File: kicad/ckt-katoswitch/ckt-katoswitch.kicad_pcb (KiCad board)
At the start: 2 copper layers, 76.2 x 63.5 mm, 50 parts, among them J1 SM04B-SRSS, J10 SM04B-SRSS, J11 Conn_AVR_TagConnect_TC2030, J2 SM04B-SRSS, J3 SM04B-SRSS, J4 SM04B-SRSS, J5 SM04B-SRSS, J6 SM04B-SRSS, J7 SM04B-SRSS, J8 SM04B-SRSS, J9 SM04B-SRSS, Q1 ZXMS6004FF, SW1 SW_DIP_x05, U1 AP7381-33Y, U2 ATtiny861A-S

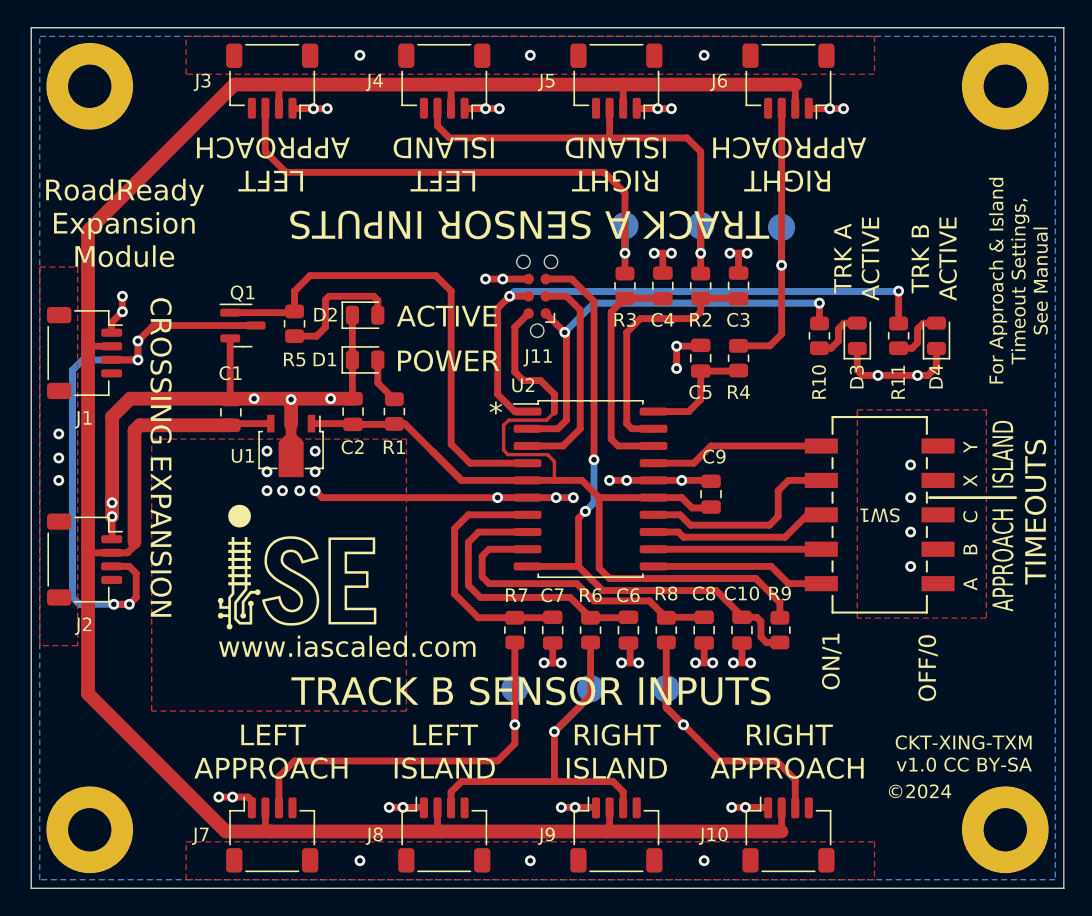
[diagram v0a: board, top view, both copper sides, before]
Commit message: Initial cut at PCB
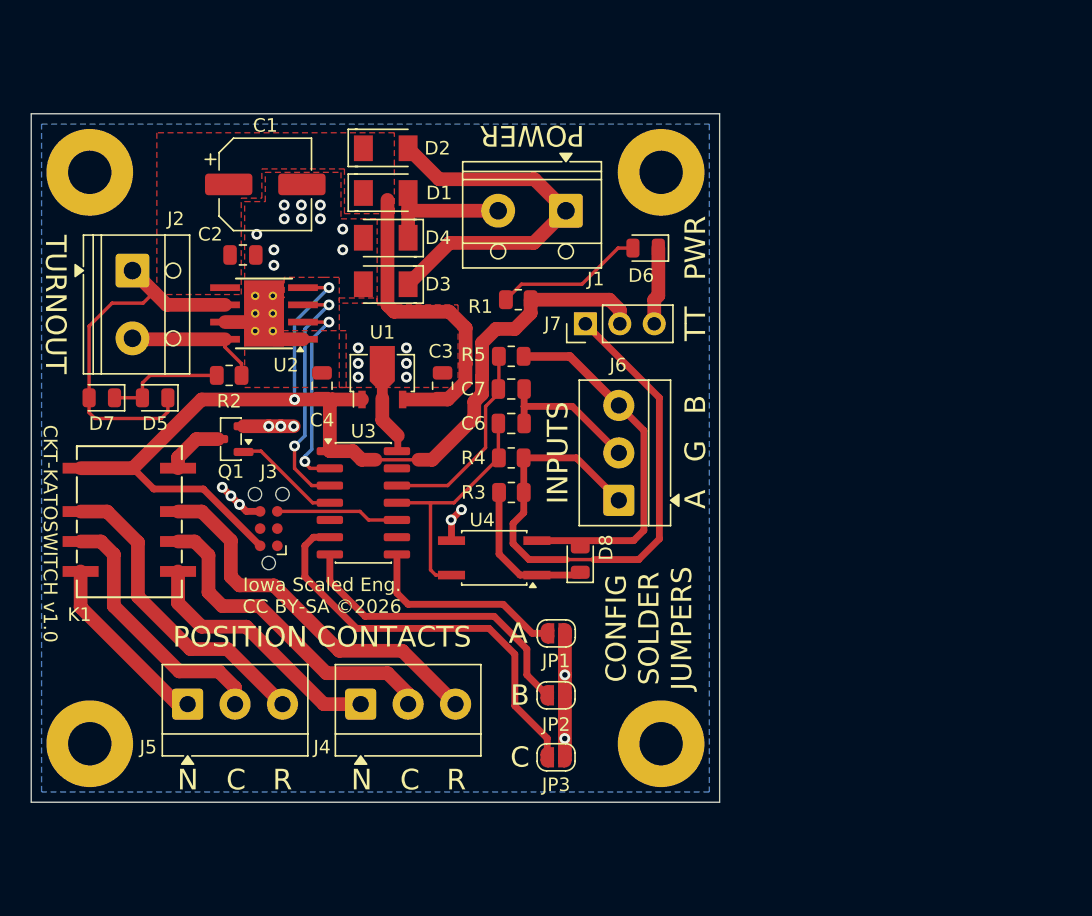
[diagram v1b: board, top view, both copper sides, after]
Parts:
- removed C10, C5, C8: 1uF, Capacitor_SMD:C_0805_2012Metric
- removed C9: 0.1uF, Capacitor_SMD:C_0805_2012Metric
- removed J10, J8, J9: SM04B-SRSS, Connector_JST:JST_SH_SM04B-SRSS-TB_1x04-1MP_P1.00mm_Horizontal
- removed J11: Conn_AVR_TagConnect_TC2030, Connector:Tag-Connect_TC2030-IDC-NL_2x03_P1.27mm_Vertical
- removed R10, R11, R6, R7, R8: 1k, Resistor_SMD:R_0805_2012Metric
- removed R9: 10k, Resistor_SMD:R_0805_2012Metric
- removed SW1: SW_DIP_x05, ISE_UltraLibrarian:CST_219SMT
- removed TP1, TP2, TP3, TP4, TP5, TP6: TestPoint, TestPoint:TestPoint_Pad_D2.0mm
- added D5: AMBER, LED_SMD:LED_0805_2012Metric, F.Cu at (34.5, 46.4)
- added D6: GREEN LED, LED_SMD:LED_0805_2012Metric, F.Cu at (70.7, 35.3)
- added D7: BLUE, LED_SMD:LED_0805_2012Metric, F.Cu at (30.6, 46.4)
- added D8: AMBER, LED_SMD:LED_0805_2012Metric, F.Cu at (65.9, 58.3)
- added JP1: SolderJumper_2_Open, Jumper:SolderJumper-2_P1.3mm_Open_RoundedPad1.0x1.5mm, F.Cu at (64.1, 63.7)
- added JP2: SolderJumper_2_Open, Jumper:SolderJumper-2_P1.3mm_Open_RoundedPad1.0x1.5mm, F.Cu at (64.1, 68.3)
- added JP3: SolderJumper_2_Open, Jumper:SolderJumper-2_P1.3mm_Open_RoundedPad1.0x1.5mm, F.Cu at (64.1, 72.9)
- added K1: AGQ200A4H, ISE_UltraLibrarian:RELAY_AGQ_A_PAN, F.Cu at (32.6, 55.5)
- added U3: ATtiny414-SS, Package_SO:SOIC-14_3.9x8.7mm_P1.27mm, F.Cu at (49.9, 54.1)
- added U4: LTV-357T, Package_SO:SO-4_4.4x3.6mm_P2.54mm, F.Cu at (59.6, 58.2)
- C1: value 10uF -> 68uF; footprint Capacitor_SMD:C_0805_2012Metric -> Capacitor_SMD:CP_Elec_6.3x5.8
- C2: value 22uF -> 10uF
- C4: value 1uF -> 22uF
- D1: value GREEN LED -> CDBM140G; footprint LED_SMD:LED_0805_2012Metric -> ISE_Generic:SOD-123T
- D2: value RED -> CDBM140G; footprint LED_SMD:LED_0805_2012Metric -> ISE_Generic:SOD-123T
- D3, D4: value AMBER -> CDBM140G; footprint LED_SMD:LED_0805_2012Metric -> ISE_Generic:SOD-123T
- J1, J2: value SM04B-SRSS -> Screw_Terminal_01x02; footprint Connector_JST:JST_SH_SM04B-SRSS-TB_1x04-1MP_P1.00mm_Horizontal -> TerminalBlock_RND:TerminalBlock_RND_205-00012_1x02_P5.00mm_Horizontal
- J3: value SM04B-SRSS -> Conn_AVR_TagConnect_TC2030; footprint Connector_JST:JST_SH_SM04B-SRSS-TB_1x04-1MP_P1.00mm_Horizontal -> Connector:Tag-Connect_TC2030-IDC-NL_2x03_P1.27mm_Vertical
- J4, J5, J6: value SM04B-SRSS -> Screw_Terminal_01x02; footprint Connector_JST:JST_SH_SM04B-SRSS-TB_1x04-1MP_P1.00mm_Horizontal -> TerminalBlock_MetzConnect:TerminalBlock_MetzConnect_Type059_RT06303HBWC_1x03_P3.50mm_Horizontal
- J7: value SM04B-SRSS -> Conn_01x03; footprint Connector_JST:JST_SH_SM04B-SRSS-TB_1x04-1MP_P1.00mm_Horizontal -> Connector_PinHeader_2.54mm:PinHeader_1x03_P2.54mm_Vertical
- Q1: value ZXMS6004FF -> DRDC3105-7
- U1: value AP7381-33Y -> AP7381-50Y
- U2: value ATtiny861A-S -> DRV8231A; footprint Package_SO:SOIC-20W_7.5x12.8mm_P1.27mm -> Package_SO:Texas_HTSOP-8-1EP_3.9x4.9mm_P1.27mm_EP2.95x4.9mm_Mask2.4x3.1mm_ThermalVias
- moved H2 67.9 mm to (29.7, 71.9)
- moved H4 64.3 mm to (71.9, 29.7)
- moved J5 55.8 mm to (36.9, 69.0), turned to 0 degrees
- moved H3 54.8 mm to (71.9, 71.9)
- moved J4 46.4 mm to (49.7, 69.0), turned to 0 degrees
- moved J7 44.2 mm to (66.3, 40.9), turned to 90 degrees
- moved D4 41.3 mm to (51.6, 34.5), turned to 180 degrees
- moved J1 37.0 mm to (64.9, 32.6), turned to 180 degrees
- moved R2 35.4 mm to (40.0, 44.7), turned to 0 degrees
- moved D3 35.0 mm to (51.6, 38.0), turned to 180 degrees
- moved J6 33.4 mm to (68.8, 53.9), turned to 90 degrees
- moved J3 33.0 mm to (42.9, 56.0), turned to 90 degrees
- moved U2 27.4 mm to (42.6, 40.1), turned to 180 degrees
- moved C4 26.2 mm to (46.9, 45.5)
- moved C3 23.1 mm to (55.8, 45.5)
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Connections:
- C2 pad 1: +3.3V -> /VIN
- C3 pad 1: /~{ISLAND_1} -> /VIN
- C4 pad 1: /~{APPR_A_1} -> +5V
- C6 pad 1: /~{ISLAND_2} -> Net-(U3-PA1)
- C7 pad 1: /~{APPR_A_2} -> Net-(U3-PA2)
- D1 pad 1: GND -> /VIN
- D1 pad 2: Net-(D1-Pad2) -> Net-(D1-A)
- D2 pad 1: GND -> /VIN
- D2 pad 2: Net-(D2-Pad2) -> Net-(D2-A)
- D3 pad 1: GND -> Net-(D2-A)
- D3 pad 2: Net-(D3-Pad2) -> GND
- D4 pad 1: GND -> Net-(D1-A)
- D4 pad 2: Net-(D4-Pad2) -> GND
- J1 pad 1: GND -> Net-(D2-A)
- J1 pad 2: /VIN -> Net-(D1-A)
- J2 pad 1: GND -> Net-(D5-K)
- J2 pad 2: /VIN -> Net-(J2-Pin_2)
- J3 pad 1: GND -> unconnected-(J3-MISO-Pad1)
- J3 pad 2: /VIN -> +5V
- J3 pad 3: Net-(J3-Pad3) -> unconnected-(J3-SCK-Pad3)
- J4 pad 1: GND -> Net-(J4-Pin_1)
- J4 pad 2: /VIN -> Net-(J4-Pin_2)
- J4 pad 3: Net-(R2-Pad1) -> Net-(J4-Pin_3)
- J5 pad 1: GND -> Net-(J5-Pin_1)
- J5 pad 2: /VIN -> Net-(J5-Pin_2)
- J5 pad 3: Net-(R2-Pad1) -> Net-(J5-Pin_3)
- J6 pad 1: GND -> Net-(J6-Pin_1)
- J6 pad 2: /VIN -> GND
- J6 pad 3: Net-(J6-Pad3) -> Net-(D8-A)
- J7 pad 1: GND -> Net-(J6-Pin_1)
- J7 pad 2: /VIN -> +5V
- J7 pad 3: Net-(J7-Pad3) -> GND
- Q1 pad 1: /~{ENABLE} -> Net-(Q1-G)
- Q1 pad 3: Net-(J1-Pad3) -> Net-(Q1-D)
- R1 pad 1: Net-(D1-Pad2) -> Net-(D6-A)
- R1 pad 2: +3.3V -> +5V
- R2 pad 1: Net-(R2-Pad1) -> Net-(D5-A)
- R2 pad 2: /~{ISLAND_1} -> Net-(J2-Pin_2)
- R3 pad 1: Net-(J3-Pad3) -> Net-(D8-K)
- R3 pad 2: /~{APPR_A_1} -> Net-(J6-Pin_1)
- R4 pad 1: Net-(J6-Pad3) -> Net-(U3-PA1)
- R4 pad 2: /~{APPR_B_1} -> Net-(J6-Pin_1)
- R5 pad 1: Net-(D2-Pad2) -> Net-(U3-PA2)
- R5 pad 2: /~{ENABLE} -> Net-(D8-A)
- U1 pad 1: +3.3V -> +5V
- U2 pad 1: /AVR_MOSI -> GND
- U2 pad 2: /AVR_MISO -> Net-(U2-IN2)
- U2 pad 3: /AVR_SCK -> Net-(U2-IN1)
- U2 pad 4: /~{ENABLE} -> +5V
- U2 pad 5: +3.3V -> /VIN
- U2 pad 6: GND -> Net-(D5-K)
- U2 pad 7: /~{APPR_A_2} -> GND
- U2 pad 8: /~{ISLAND_2} -> Net-(J2-Pin_2)
- U2 pad 9: /~{APPR_B_2} -> GND
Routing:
- net /VIN: track 184.8 -> 23.1 mm
- net +5V: track 0.00 -> 81.1 mm, vias 0 -> 2
- net +3.3V: track 77.0 -> 0.00 mm
- net GND: track 123.3 -> 47.5 mm, vias 68 -> 27
- net /~{RESET}: track 45.9 -> 0.00 mm, vias 2 -> 0
- net Net-(J1-Pad3): track 45.9 -> 0.00 mm, vias 4 -> 0
- net Net-(J6-Pin_1): track 0.00 -> 45.0 mm
- net /AVR_MOSI: track 43.0 -> 0.00 mm, vias 2 -> 0
- net Net-(J3-Pad3): track 39.0 -> 0.00 mm, vias 1 -> 0
- net /~{ENABLE}: track 36.3 -> 0.00 mm
- net Net-(R2-Pad1): track 34.7 -> 0.00 mm, vias 1 -> 0
- net /AVR_MISO: track 32.8 -> 0.00 mm, vias 2 -> 0
- net Net-(J8-Pad3): track 31.3 -> 0.00 mm, vias 1 -> 0
- net Net-(J7-Pad3): track 30.9 -> 0.00 mm, vias 1 -> 0
- net Net-(JP3-B): track 0.00 -> 30.8 mm
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- added copper zone on F.Cu, net /VIN
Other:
- board size 76.2 x 63.5 mm -> 50.8 x 50.8 mm
- board text added: "CKT-KATOSWITCH v1.0"
- board text added: "CONFIG SOLDER JUMPERS"
- board text added: "G"
- board text added: "INPUTS"
- board text added: "Iowa Scaled Eng. CC BY-SA ©2026"
- board text added: "N"
- board text added: "POSITION CONTACTS"
- board text added: "PWR"
- board text added: "R"
- board text added: "TT"
- board text added: "TURNOUT"
- board text removed: "*"
- board text removed: "ACTIVE"
- board text removed: "APPROACH"
- board text removed: "CKT-XING-TXM v1.0 CC BY-SA"
- board text removed: "CROSSING EXPANSION"
- board text removed: "For Approach & Island Timeout Settings, See Manual"
- board text removed: "ISLAND"
- board text removed: "LEFT APPROACH"
- board text removed: "LEFT ISLAND"
- board text removed: "ON/1"
- board text removed: "RIGHT APPROACH"
- board text removed: "RIGHT ISLAND"
- board text removed: "RoadReady Expansion Module"
- board text removed: "TIMEOUTS"
- board text removed: "TRACK A SENSOR INPUTS"
- board text removed: "TRACK B SENSOR INPUTS"
- board text removed: "TRK A ACTIVE"
- board text removed: "TRK B ACTIVE"
- board text removed: "X"
- board text removed: "Y"
- board text removed: "www.iascaled.com"
- board text removed: "©2024"
